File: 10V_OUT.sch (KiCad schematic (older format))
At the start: 7 parts, among them U1 LM321

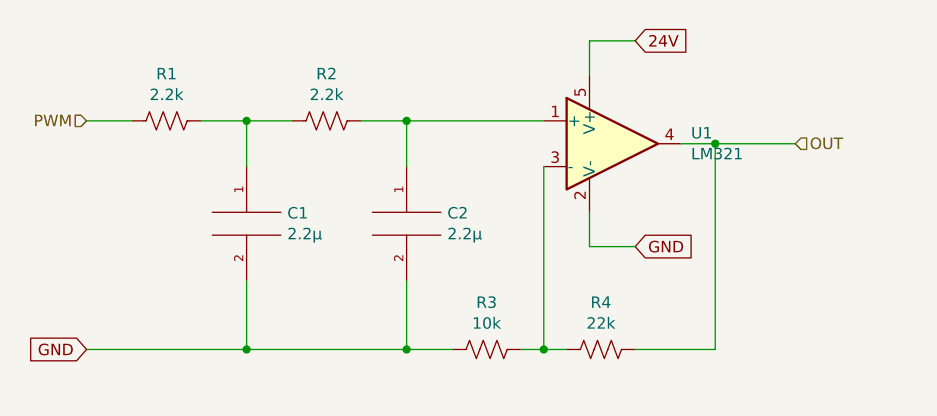
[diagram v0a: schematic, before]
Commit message: Comments and Notation for clarity
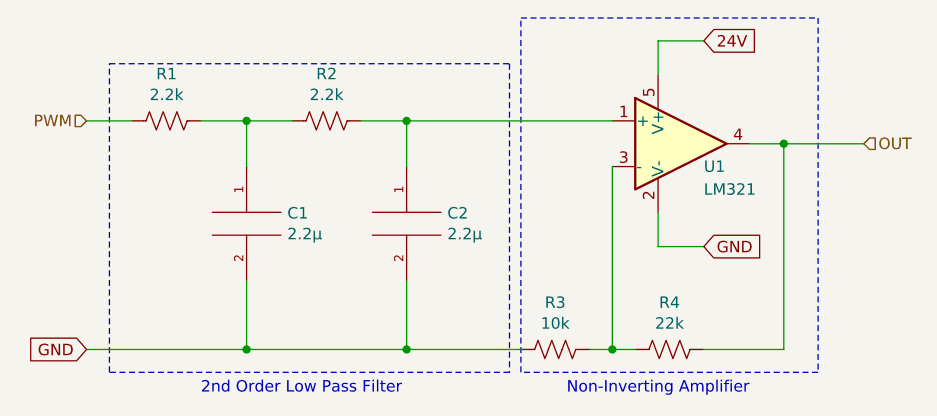
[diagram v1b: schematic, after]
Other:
- note added: "2nd Order Low Pass Filter"
- note added: "Non-Inverting Amplifier"
- moved on the sheet: R3, R4, U1
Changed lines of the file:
@@
 L Amplifier_Operational:LM321 U1
 U 1 1 60A73539
-P 6850 3450
-F 0 "U1" H 7194 3496 50  0000 L CNN
-F 1 "LM321" H 7194 3405 50  0000 L CNN
-F 2 "Package_TO_SOT_SMD:SOT-23-5" H 6850 3450 50  0001 C CNN
-F 3 "http://www.ti.com/lit/ds/symlink/lm321.pdf" H 6850 3450 50  0001 C CNN
-	1    6850 3450
+P 7150 3450
+F 0 "U1" H 7250 3350 50  0000 L CNN
+F 1 "LM321" H 7250 3250 50  0000 L CNN
+F 2 "Package_TO_SOT_SMD:SOT-23-5" H 7150 3450 50  0001 C CNN
+F 3 "http://www.ti.com/lit/ds/symlink/lm321.pdf" H 7150 3450 50  0001 C CNN
+	1    7150 3450
 	1    0    0    -1
 $EndComp
@@
 L Device:R_US R4
 U 1 1 60A77E98
-P 6800 4350
-F 0 "R4" V 6595 4350 50  0000 C CNN
-F 1 "22k" V 6686 4350 50  0000 C CNN
-F 2 "" V 6840 4340 50  0001 C CNN
-F 3 "~" H 6800 4350 50  0001 C CNN
-	1    6800 4350
+P 7100 4350
+F 0 "R4" V 6895 4350 50  0000 C CNN
+F 1 "22k" V 6986 4350 50  0000 C CNN
+F 2 "" V 7140 4340 50  0001 C CNN
+F 3 "~" H 7100 4350 50  0001 C CNN
+	1    7100 4350
 	0    1    1    0
 $EndComp
@@
 L Device:R_US R3
 U 1 1 60A78F26
-P 6300 4350
-F 0 "R3" V 6095 4350 50  0000 C CNN
-F 1 "10k" V 6186 4350 50  0000 C CNN
-F 2 "" V 6340 4340 50  0001 C CNN
-F 3 "~" H 6300 4350 50  0001 C CNN
-	1    6300 4350
+P 6600 4350
+F 0 "R3" V 6395 4350 50  0000 C CNN
+F 1 "10k" V 6486 4350 50  0000 C CNN
+F 2 "" V 6640 4340 50  0001 C CNN
+F 3 "~" H 6600 4350 50  0001 C CNN
+	1    6600 4350
 	0    1    1    0
 $EndComp
@@
 	5950 3350 5950 3550
 Wire Wire Line
-	5950 3350 6550 3350
-Connection ~ 5950 3350
+	7450 3450 7600 3450
 Wire Wire Line
-	7150 3450 7300 3450
+	7600 3450 7600 4350
 Wire Wire Line
-	7300 3450 7300 4350
+	7600 4350 7250 4350
 Wire Wire Line
-	7300 4350 6950 4350
+	6950 4350 6850 4350
 Wire Wire Line
-	6650 4350 6550 4350
+	6850 3550 6850 4350
+Connection ~ 6850 4350
 Wire Wire Line
-	6550 3550 6550 4350
-Connection ~ 6550 4350
-Wire Wire Line
-	6550 4350 6450 4350
-Wire Wire Line
-	6150 4350 5950 4350
+	6850 4350 6750 4350
 Wire Wire Line
 	5250 4050 5250 4350
@@
 Wire Wire Line
 	5950 4050 5950 4350
+Wire Wire Line
+	5950 4350 5250 4350
+Text HLabel 7950 3450 2    50   Input ~ 0
+OUT
+Wire Wire Line
+	7600 3450 7950 3450
+Connection ~ 7600 3450
+Text GLabel 7250 3900 2    50   Input ~ 0
+GND
+Wire Wire Line
+	7050 3750 7050 3900
+Wire Wire Line
+	7050 3900 7250 3900
+Text GLabel 7250 3000 2    50   Input ~ 0
+24V
+Wire Wire Line
+	7050 3150 7050 3000
+Wire Wire Line
+	7050 3000 7250 3000
+Wire Wire Line
+	5950 4350 6450 4350
 Connection ~ 5950 4350
 Wire Wire Line
-	5950 4350 5250 4350
-Text HLabel 7650 3450 2    50   Input ~ 0
-OUT
-Wire Wire Line
-	7300 3450 7650 3450
-Connection ~ 7300 3450
-Text GLabel 6950 3900 2    50   Input ~ 0
-GND
-Wire Wire Line
-	6750 3750 6750 3900
-Wire Wire Line
-	6750 3900 6950 3900
-Text GLabel 6950 3000 2    50   Input ~ 0
-24V
-Wire Wire Line
-	6750 3150 6750 3000
-Wire Wire Line
-	6750 3000 6950 3000
+	6850 3350 5950 3350
+Connection ~ 5950 3350
+Wire Notes Line
+	4650 3100 6400 3100
+Wire Notes Line
+	6400 3100 6400 4450
+Wire Notes Line
+	6400 4450 4650 4450
+Wire Notes Line
+	4650 4450 4650 3100
+Text Notes 5050 4550 0    50   ~ 0
+2nd Order Low Pass Filter
+Wire Notes Line
+	6450 2900 7750 2900
+Wire Notes Line
+	7750 2900 7750 4450
+Wire Notes Line
+	7750 4450 6450 4450
+Wire Notes Line
+	6450 4450 6450 2900
+Text Notes 6650 4550 0    50   ~ 0
+Non-Inverting Amplifier
 $EndSCHEMATC
